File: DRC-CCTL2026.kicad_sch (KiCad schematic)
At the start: 46 parts, among them J1 USB_C, J10 SW3, J2 FDCAN1, J3 FDCAN2, J4 FDCAN3, J5 SW1, J6 SW2, J7 STLINK, J8 I2C, J9 USART, Q1 MMBT3904, SW1 SW_Push, SW2 DIP, U1 STM32G474RETx, U2 AZ1084C-3.3, U3 74AHC1G125, Y1 8M10PB/XT324-10/80

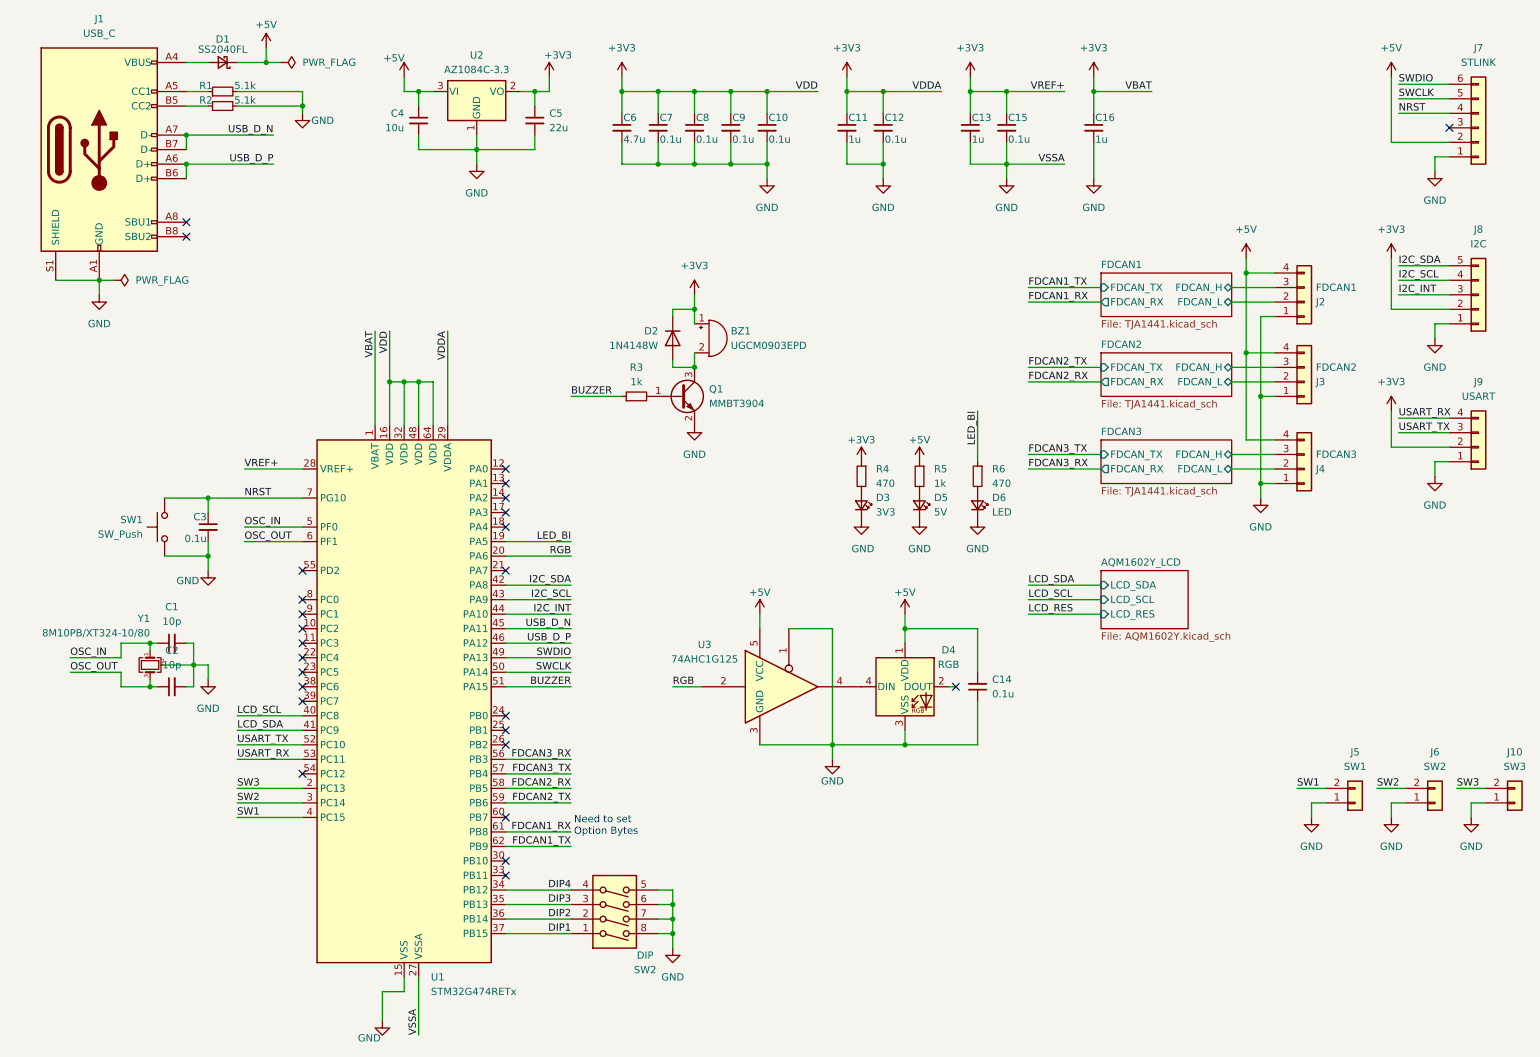
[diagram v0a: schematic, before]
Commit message: v0.2.0
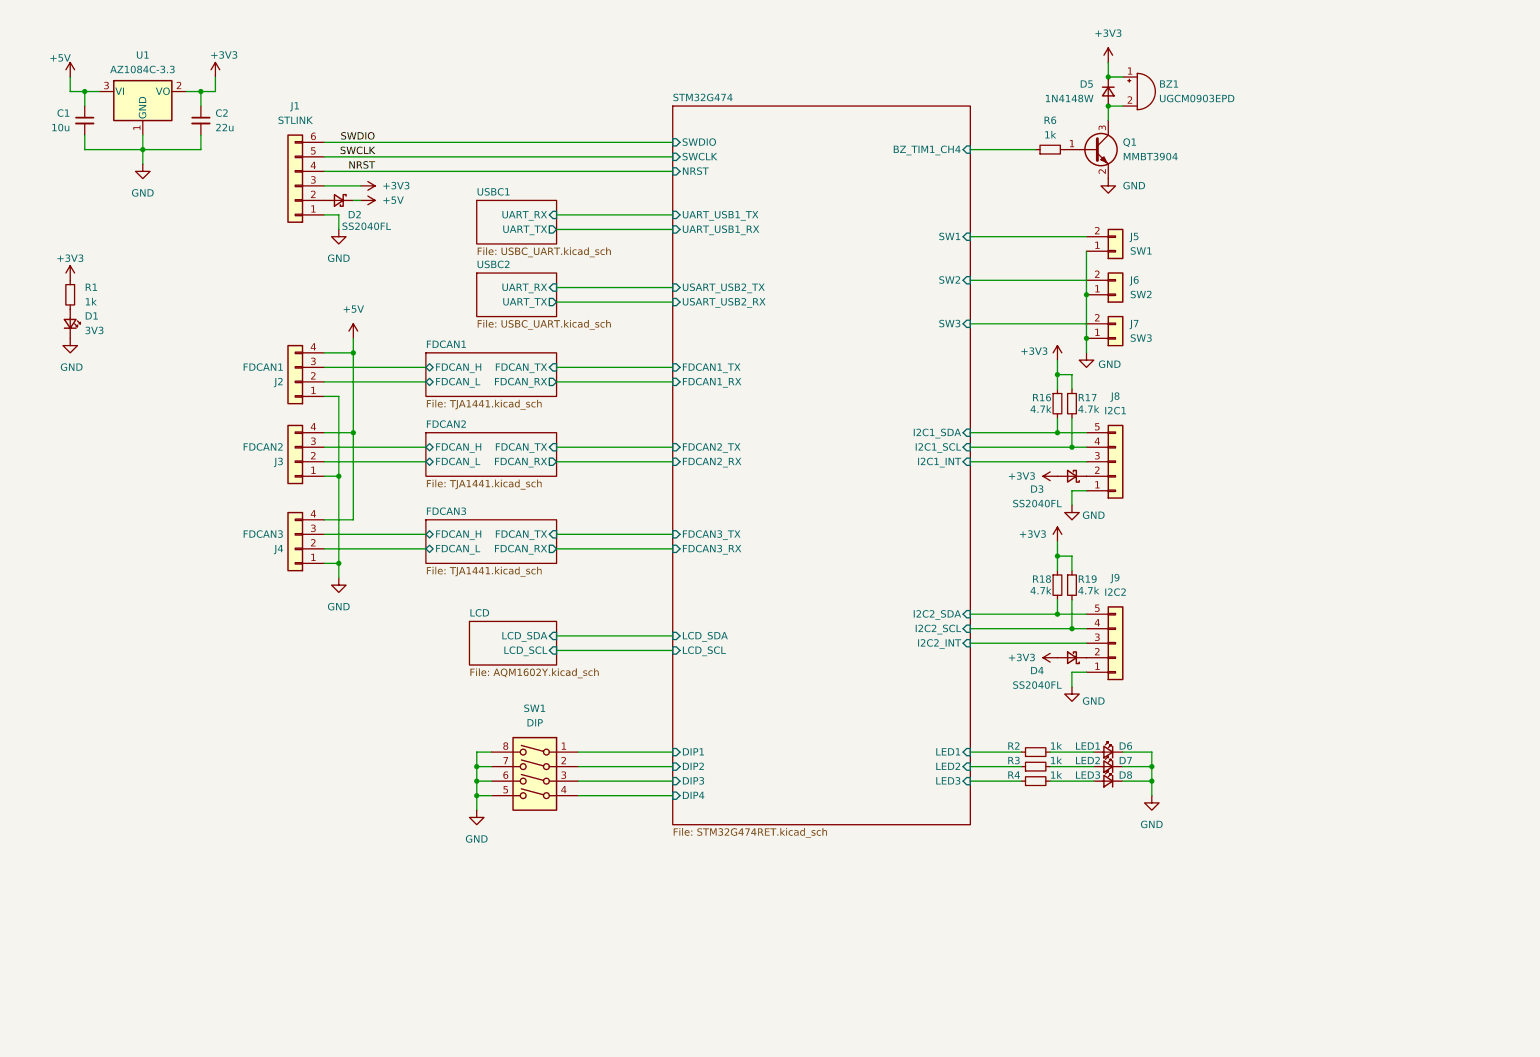
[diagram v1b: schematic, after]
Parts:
- removed C1, C2: 10p, Capacitor_THT:C_Disc_D5.0mm_W2.5mm_P5.00mm, symbol Device:C_Small
- removed C10, C12, C14, C15, C3, C7, C8, C9: 0.1u, Capacitor_SMD:C_0603_1608Metric_Pad1.08x0.95mm_HandSolder, symbol Device:C_Small
- removed C11, C13, C16: 1u, Capacitor_SMD:C_0603_1608Metric_Pad1.08x0.95mm_HandSolder, symbol Device:C_Small
- removed C6: 4.7u, Capacitor_SMD:C_0805_2012Metric_Pad1.18x1.45mm_HandSolder, symbol Device:C_Small
- removed D1: SS2040FL, Diode_SMD:D_SOD-123F, symbol Device:D_Schottky_Small
- removed D2: 1N4148W, Diode_SMD:D_SOD-123, symbol Diode:1N4148W
- removed D4: RGB, LED_SMD:LED_WS2812B_PLCC4_5.0x5.0mm_P3.2mm, symbol LED:WS2812B
- removed D5: 5V, LED_SMD:LED_0603_1608Metric_Pad1.05x0.95mm_HandSolder, symbol Device:LED_Small
- removed J1: USB_C, Connector_USB:USB_C_Receptacle_GCT_USB4105-xx-A_16P_TopMnt_Horizontal, symbol Connector:USB_C_Receptacle_USB2.0_16P
- removed J9: USART, Connector_JST:JST_XH_S4B-XH-A_1x04_P2.50mm_Horizontal, symbol Connector_Generic:Conn_01x04
- removed R1: 5.1k, Resistor_SMD:R_0603_1608Metric_Pad0.98x0.95mm_HandSolder, symbol lib:R_Small
- removed R5: 1k, Resistor_SMD:R_0603_1608Metric_Pad0.98x0.95mm_HandSolder, symbol lib:R_Small
- removed R6: 470, Resistor_SMD:R_0603_1608Metric_Pad0.98x0.95mm_HandSolder, symbol lib:R_Small
- removed SW1: SW_Push, Button_Switch_SMD:SW_SPST_EVQPE1, symbol Switch:SW_Push
- removed U1: STM32G474RETx, Package_QFP:LQFP-64_10x10mm_P0.5mm, symbol MCU_ST_STM32G4:STM32G474RETx
- removed U3: 74AHC1G125, Package_TO_SOT_SMD:SOT-353_SC-70-5, symbol 74xGxx:74AHC1G125
- removed Y1: 8M10PB/XT324-10/80, lib:8M10PB_XT324-10_80, symbol Device:Crystal_GND24_Small
- added D2, D3, D4: SS2040FL, Diode_SMD:D_SOD-123F, symbol Device:D_Schottky_Small
- added D5: 1N4148W, Diode_SMD:D_SOD-123, symbol Device:D_Small
- added D7: LED2, LED_SMD:LED_0603_1608Metric_Pad1.05x0.95mm_HandSolder, symbol Device:LED_Small
- added D8: LED3, LED_SMD:LED_0603_1608Metric_Pad1.05x0.95mm_HandSolder, symbol Device:LED_Small
- added J9: I2C2, Connector_JST:JST_XH_S5B-XH-A_1x05_P2.50mm_Horizontal, symbol Connector_Generic:Conn_01x05
- added R16, R17, R18, R19: 4.7k, Resistor_SMD:R_0603_1608Metric_Pad0.98x0.95mm_HandSolder, symbol lib:R_Small
- added R3, R4: 1k, Resistor_SMD:R_0603_1608Metric_Pad0.98x0.95mm_HandSolder, symbol lib:R_Small
- D6: value LED -> LED1
- J1: renamed from J7; footprint Connector_JST:JST_PH_S6B-PH-K_1x06_P2.00mm_Horizontal -> Connector_IDC:IDC-Header_2x03_P2.54mm_Vertical
- J8: value I2C -> I2C1
- R1: renamed from R4; value 470 -> 1k
- R2: value 5.1k -> 1k
- renumbered C4 to C1, C5 to C2, D3 to D1, J10 to J7, R3 to R6, SW2 to SW1, U2 to U1
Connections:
- net +3V3: now also J1.3 (Pin_3), D3.2 (A), D4.2 (A), D5.1 (K), R16.1, R17.1, R18.1, R19.1; no longer J8.2 (Pin_2)
- net +5V: now also D2.1 (K); no longer J1.2 (Pin_2)
- net GND: now also D7.1 (K), D8.1 (K), J9.1 (Pin_1); no longer R2.2
- net STM32G474/LED1: now reaches R2.1
- net at D6.2 (A): now also R2.2
- net at BZ1.2 (-), Q1.3 (C): now also D5.2 (A)
- net BUZZER renamed STM32G474/BZ_TIM1_CH4
- net DIP1 renamed STM32G474/DIP1
- net DIP2 renamed STM32G474/DIP2
- net DIP3 renamed STM32G474/DIP3
- net DIP4 renamed STM32G474/DIP4
- net I2C_INT renamed STM32G474/I2C1_INT
- net I2C_SCL renamed STM32G474/I2C1_SCL
- net STM32G474/I2C1_SCL: now also R17.2
- net I2C_SDA renamed STM32G474/I2C1_SDA
- net STM32G474/I2C1_SDA: now also R16.2
- net SW1 renamed STM32G474/SW1
- net SW2 renamed STM32G474/SW2
- net SW3 renamed STM32G474/SW3
- new net: D3.1 (K), J8.2 (Pin_2)
- new net: D2.2 (A), J1.2 (Pin_2)
- new net: D8.2 (A), R4.2
- new net: D7.2 (A), R3.2
- new net: D4.1 (K), J9.2 (Pin_2)
- new net STM32G474/I2C2_INT: J9.3 (Pin_3)
- new net STM32G474/I2C2_SCL: J9.4 (Pin_4), R19.2
- new net STM32G474/I2C2_SDA: J9.5 (Pin_5), R18.2
- new net STM32G474/LED2: R3.1
- new net STM32G474/LED3: R4.1
- no-connect marks 26 -> 0
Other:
- sheet AQM1602Y_LCD renamed LCD
- added sheet STM32G474 (STM32G474RET.kicad_sch)
- added sheet USBC1 (USBC_UART.kicad_sch)
- added sheet USBC2 (USBC_UART.kicad_sch)
- sheet LCD ports: added none; removed LCD_RES
- note removed: "Need to set Option Bytes"
- moved on the sheet: BZ1, C1, C2, D1, J1, J2, J3, J4, J5, J6, J7, J8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
